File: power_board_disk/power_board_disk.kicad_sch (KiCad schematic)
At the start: 21 parts, among them J2 Conn_01x03_Pin, J3 Screw_Terminal_01x03, J4 Screw_Terminal_01x03, U1 LMC6082, U3 REF3025, U5 INA159AIDGKR

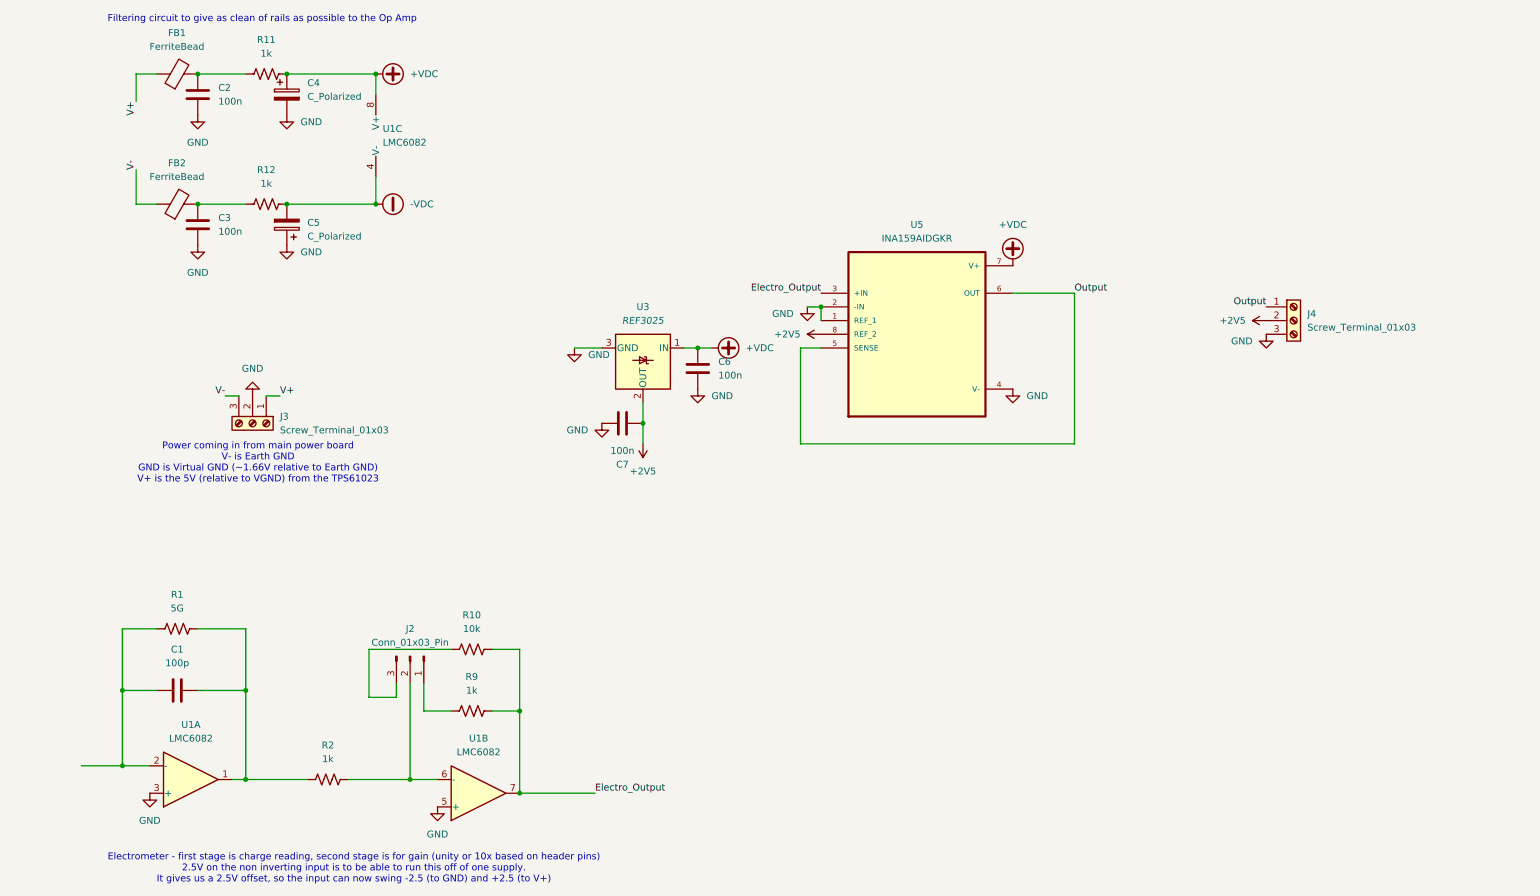
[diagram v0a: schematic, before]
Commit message: perfunctory commit
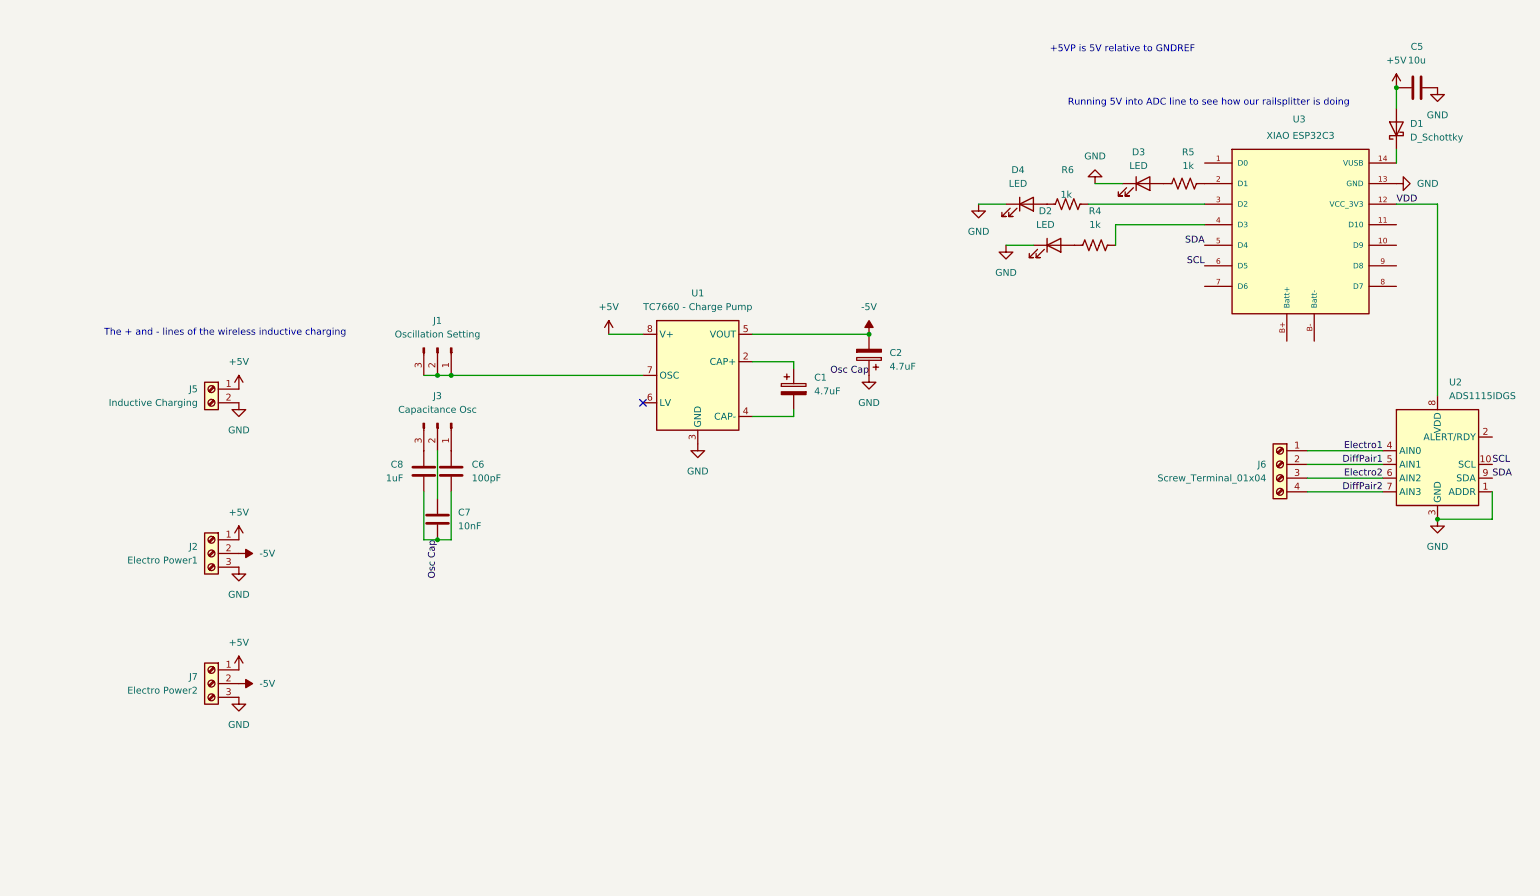
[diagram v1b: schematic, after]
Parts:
- removed C1: 100p, Capacitor_THT:C_Disc_D3.0mm_W1.6mm_P2.50mm, symbol Device:C
- removed C2, C3: 100n, Capacitor_SMD:C_1206_3216Metric, symbol Device:C
- removed C4, C5: C_Polarized, Capacitor_SMD:CP_Elec_10x10.5, symbol Device:C_Polarized
- removed FB1, FB2: FerriteBead, Inductor_SMD:L_1206_3216Metric, symbol Device:FerriteBead
- removed J2: Conn_01x03_Pin, Connector_PinHeader_2.54mm:PinHeader_1x03_P2.54mm_Vertical, symbol Connector:Conn_01x03_Pin
- removed J3, J4: Screw_Terminal_01x03, TerminalBlock_MetzConnect:TerminalBlock_MetzConnect_Type055_RT01503HDWU_1x03_P5.00mm_Horizontal, symbol Connector:Screw_Terminal_01x03
- removed R1: 5G, Resistor_THT:R_Axial_DIN0204_L3.6mm_D1.6mm_P2.54mm_Vertical, symbol Device:R_US
- removed R10: 10k, Resistor_SMD:R_1206_3216Metric_Pad1.30x1.75mm_HandSolder, symbol Device:R_US
- removed R11, R12, R2, R9: 1k, Resistor_SMD:R_1206_3216Metric_Pad1.30x1.75mm_HandSolder, symbol Device:R_US
- removed U1: LMC6082, Package_DIP:DIP-8_W7.62mm, symbol Amplifier_Operational:LMC6082
- removed U3: REF3025, Package_TO_SOT_SMD:SOT-23, symbol Reference_Voltage:REF3025
- removed U5: INA159AIDGKR, Package_SO:TSSOP-8_3x3mm_P0.65mm, symbol ADS8681:INA159AIDGKR
- added C1, C2: 4.7uF, Capacitor_Tantalum_SMD:CP_EIA-3216-18_Kemet-A_HandSolder, symbol Device:C_Polarized
- added C5: 10u, Capacitor_SMD:C_1206_3216Metric_Pad1.33x1.80mm_HandSolder, symbol Device:C
- added C8: 1uF, Capacitor_SMD:C_1206_3216Metric_Pad1.33x1.80mm_HandSolder, symbol Device:C
- added D1: D_Schottky, Diode_THT:D_A-405_P7.62mm_Horizontal, symbol Device:D_Schottky
- added D2, D3, D4: LED, LED_THT:LED_D1.8mm_W3.3mm_H2.4mm, symbol Device:LED
- added J1: Oscillation Setting, Connector_PinHeader_2.54mm:PinHeader_1x03_P2.54mm_Vertical, symbol Connector:Conn_01x03_Pin
- added J2: Electro Power1, TerminalBlock_MetzConnect:TerminalBlock_MetzConnect_Type055_RT01503HDWU_1x03_P5.00mm_Horizontal, symbol Connector:Screw_Terminal_01x03
- added J3: Capacitance Osc, Connector_PinHeader_2.54mm:PinHeader_1x03_P2.54mm_Vertical, symbol Connector:Conn_01x03_Pin
- added J5: Inductive Charging, TerminalBlock:TerminalBlock_MaiXu_MX126-5.0-02P_1x02_P5.00mm, symbol Connector:Screw_Terminal_01x02
- added J6: Screw_Terminal_01x04, TerminalBlock_MetzConnect:TerminalBlock_MetzConnect_Type055_RT01504HDWU_1x04_P5.00mm_Horizontal, symbol Connector:Screw_Terminal_01x04
- added J7: Electro Power2, TerminalBlock_MetzConnect:TerminalBlock_MetzConnect_Type055_RT01503HDWU_1x03_P5.00mm_Horizontal, symbol Connector:Screw_Terminal_01x03
- added R4, R5, R6: 1k, Resistor_SMD:R_1206_3216Metric_Pad1.30x1.75mm_HandSolder, symbol Device:R_US
- added U1: TC7660 - Charge Pump, Package_SO:SOIC-8_3.9x4.9mm_P1.27mm, symbol Regulator_SwitchedCapacitor:LMC7660
- added U2: ADS1115IDGS, Package_SO:TSSOP-10_3x3mm_P0.5mm, symbol Analog_ADC:ADS1115IDGS
- added U3: XIAO ESP32C3, xiao:XIAO-ESP32-C6-DIP, symbol xiao_esp32c3:XIAO ESP32C3
- C6: value 100n -> 100pF; footprint Capacitor_SMD:C_1206_3216Metric -> Capacitor_SMD:C_1206_3216Metric_Pad1.33x1.80mm_HandSolder
- C7: value 100n -> 10nF; footprint Capacitor_SMD:C_1206_3216Metric -> Capacitor_SMD:C_1206_3216Metric_Pad1.33x1.80mm_HandSolder
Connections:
- net GND: now also C2.1, C5.2, C8.1, D2.1 (K), D3.1 (K), D4.1 (K), J2.3 (Pin_3), J5.2 (Pin_2), J7.3 (Pin_3), U1.3 (GND), U2.1 (ADDR), U2.3 (GND), U3.13 (GND)
- net +2V5: no longer names the net of C7.2
- net +2V5: now also J3.2 (Pin_2)
- net +VDC: no longer names the net of C6.2
- net +VDC: now also J3.1 (Pin_1)
- new net: D3.2 (A), R5.1
- new net: D4.2 (A), R6.1
- new net: D1.1 (K), U3.14 (VUSB)
- new net: R5.2, U3.2 (D1)
- new net: R6.2, U3.3 (D2)
- new net: R4.2, U3.4 (D3)
- new net: D2.2 (A), R4.1
- new net: C8.2, J3.3 (Pin_3)
- new net: J1.1 (Pin_1), J1.2 (Pin_2), J1.3 (Pin_3), U1.7 (OSC)
- new net: C1.1, U1.2 (CAP+)
- new net: C1.2, U1.4 (CAP-)
- new net +5V: C5.1, D1.2 (A), J2.1 (Pin_1), J5.1 (Pin_1), J7.1 (Pin_1), U1.8 (V+)
- new net -5V: C2.2, J2.2 (Pin_2), J7.2 (Pin_2), U1.5 (VOUT)
- new net DiffPair1: J6.2 (Pin_2), U2.5 (AIN1)
- new net DiffPair2: J6.4 (Pin_4), U2.7 (AIN3)
- new net Electro1: J6.1 (Pin_1), U2.4 (AIN0)
- new net Electro2: J6.3 (Pin_3), U2.6 (AIN2)
- new net SCL: U2.10 (SCL), U3.6 (D5)
- new net SDA: U2.9 (SDA), U3.5 (D4)
- new net VDD: U2.8 (VDD), U3.12 (VCC_3V3)
- no-connect marks 0 -> 1
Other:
- note added: "+5VP is 5V relative to GNDREF"
- note added: "Running 5V into ADC line to see how our railsplitter is doing"
- note added: "The + and - lines of the wireless inductive charging"
- note removed: "Electrometer - first stage is charge reading, second stage is for gain (unity or 10x based on header pins) 2.5V on the non inverting input is to be able to run this off of one supply. It gives us a 2.5V offset, so the input can now swing -2.5 (to GND) and +2.5 (to V+)"
- note removed: "Filtering circuit to give as clean of rails as possible to the Op Amp"
- note removed: "Power coming in from main power board V- is Earth GND GND is Virtual GND (~1.66V relative to Earth GND) V+ is the 5V (relative to VGND) from the TPS61023"
